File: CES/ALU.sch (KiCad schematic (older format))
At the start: 24 parts, among them U201 74HC02, U202 74HC02, U203 74HC02, U204 74HC02, U205 74HC283, U206 74HC283, U207 74HC283, U208 74HC283, U209 74HC257, U210 74HC257, U211 74HC257, U212 74HC257

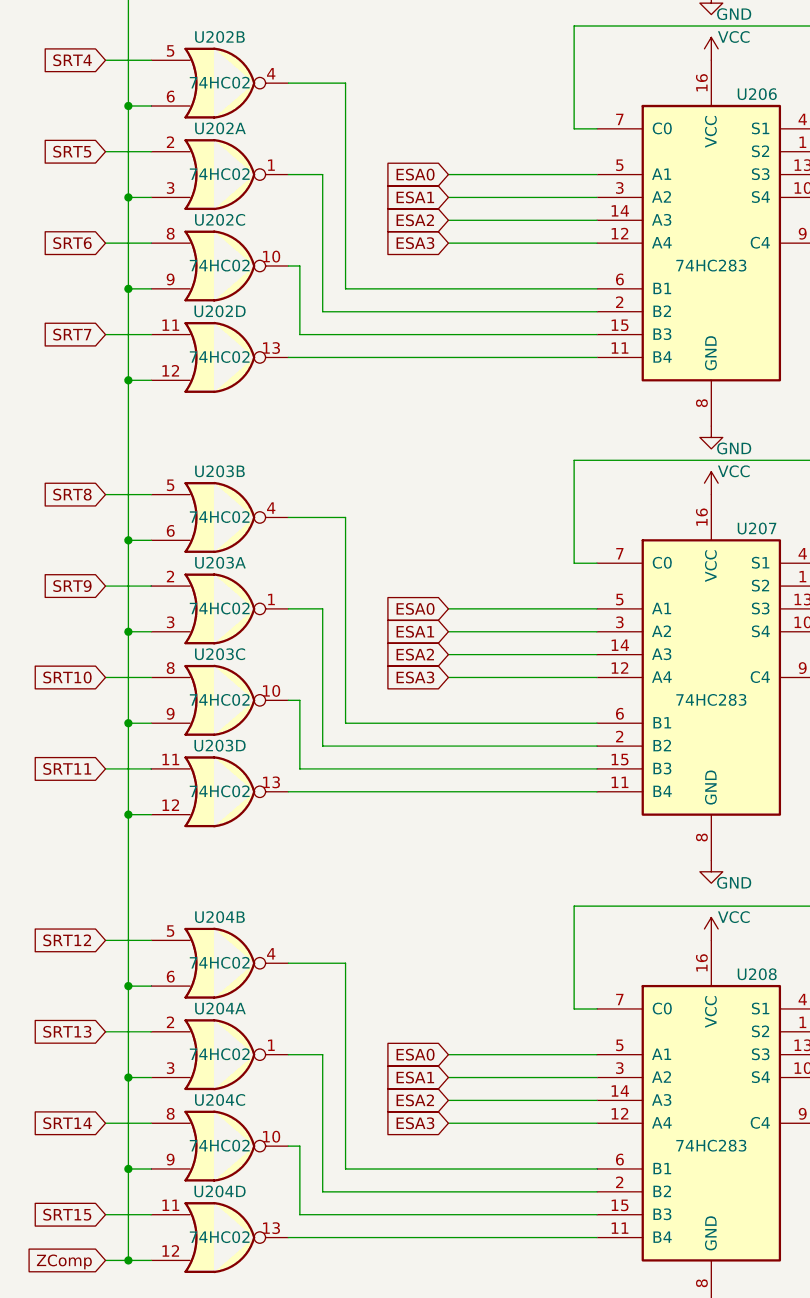
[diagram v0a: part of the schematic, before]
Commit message: Crtl+C Crlt+V
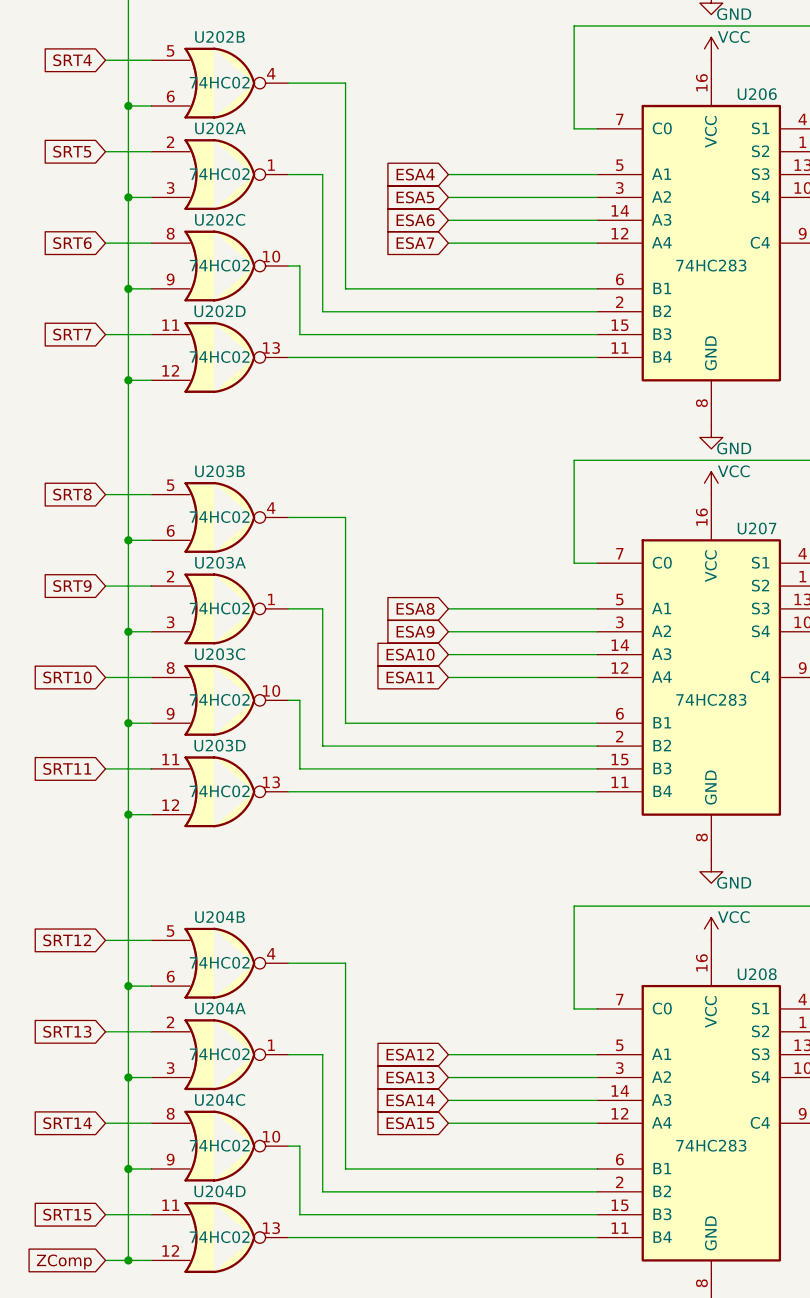
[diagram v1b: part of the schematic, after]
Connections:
- net ESA0: no longer U206.5 (A1), U207.5 (A1), U208.5 (A1)
- net ESA1: no longer U206.3 (A2), U207.3 (A2), U208.3 (A2)
- net ESA2: no longer U206.14 (A3), U207.14 (A3), U208.14 (A3)
- net ESA3: no longer U206.12 (A4), U207.12 (A4), U208.12 (A4)
- new net ESA10: U207.14 (A3)
- new net ESA11: U207.12 (A4)
- new net ESA12: U208.5 (A1)
- new net ESA13: U208.3 (A2)
- new net ESA14: U208.14 (A3)
- new net ESA15: U208.12 (A4)
- new net ESA4: U206.5 (A1)
- new net ESA5: U206.3 (A2)
- new net ESA6: U206.14 (A3)
- new net ESA7: U206.12 (A4)
- new net ESA8: U207.5 (A1)
- new net ESA9: U207.3 (A2)
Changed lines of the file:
@@
 	1850 3500 2950 3500
 Text GLabel 2300 3000 0    50   Input ~ 0
-ESA0
+ESA4
 Wire Wire Line
 	2300 3000 2950 3000
 Text GLabel 2300 3100 0    50   Input ~ 0
-ESA1
+ESA5
 Wire Wire Line
 	2300 3100 2950 3100
 Text GLabel 2300 3200 0    50   Input ~ 0
-ESA2
+ESA6
 Wire Wire Line
 	2300 3200 2950 3200
 Text GLabel 2300 3300 0    50   Input ~ 0
-ESA3
+ESA7
 Wire Wire Line
 	2300 3300 2950 3300
@@
 	1850 5400 2950 5400
 Text GLabel 2300 4900 0    50   Input ~ 0
-ESA0
+ESA8
 Wire Wire Line
 	2300 4900 2950 4900
 Text GLabel 2300 5000 0    50   Input ~ 0
-ESA1
+ESA9
 Wire Wire Line
 	2300 5000 2950 5000
 Text GLabel 2300 5100 0    50   Input ~ 0
-ESA2
+ESA10
 Wire Wire Line
 	2300 5100 2950 5100
 Text GLabel 2300 5200 0    50   Input ~ 0
-ESA3
+ESA11
 Wire Wire Line
 	2300 5200 2950 5200
@@
 	1850 7350 2950 7350
 Text GLabel 2300 6850 0    50   Input ~ 0
-ESA0
+ESA12
 Wire Wire Line
 	2300 6850 2950 6850
 Text GLabel 2300 6950 0    50   Input ~ 0
-ESA1
+ESA13
 Wire Wire Line
 	2300 6950 2950 6950
 Text GLabel 2300 7050 0    50   Input ~ 0
-ESA2
+ESA14
 Wire Wire Line
 	2300 7050 2950 7050
 Text GLabel 2300 7150 0    50   Input ~ 0
-ESA3
+ESA15
 Wire Wire Line
 	2300 7150 2950 7150
